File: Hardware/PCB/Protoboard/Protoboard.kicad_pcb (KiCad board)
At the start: 2 copper layers, 17 parts, among them J1 Conn_01x05_Female, J2 Conn_01x08_Female, J3 Conn_01x08_Female, U1 MAX6971ANG_

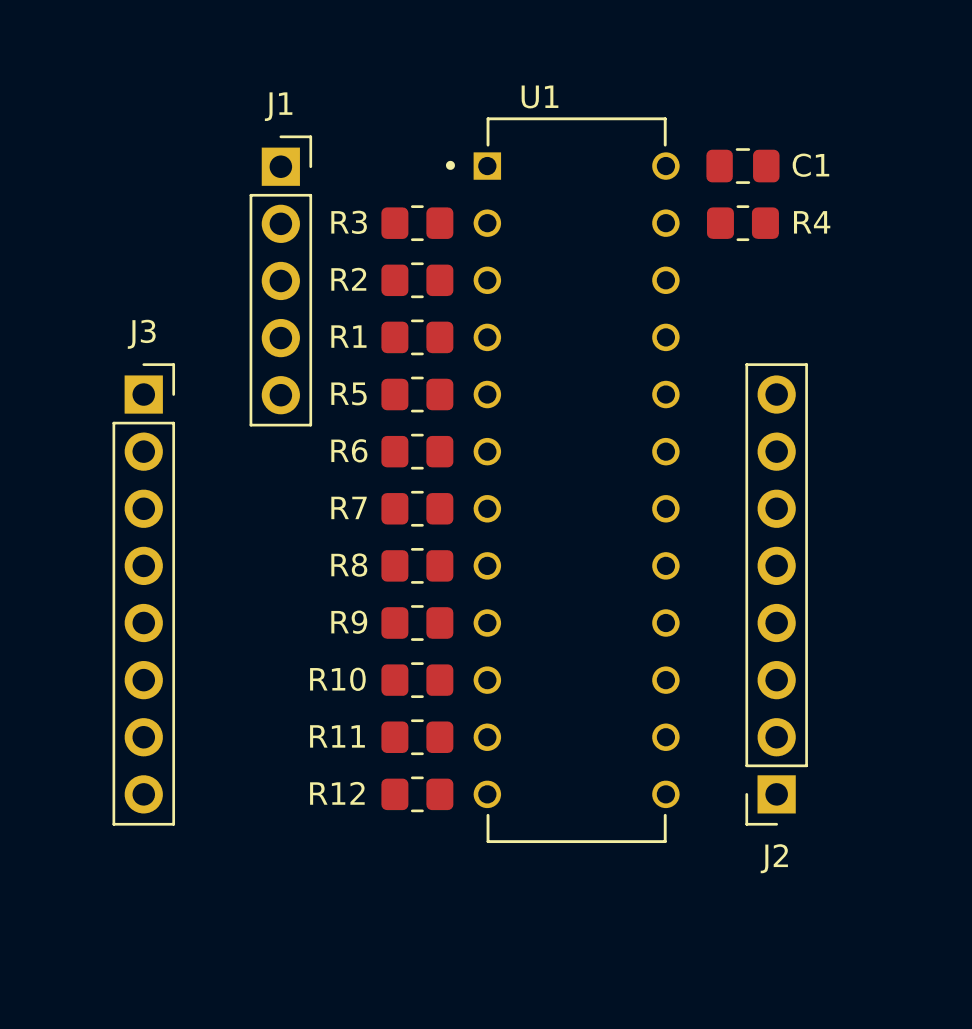
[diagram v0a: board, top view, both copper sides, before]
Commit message: Finished Protoboard
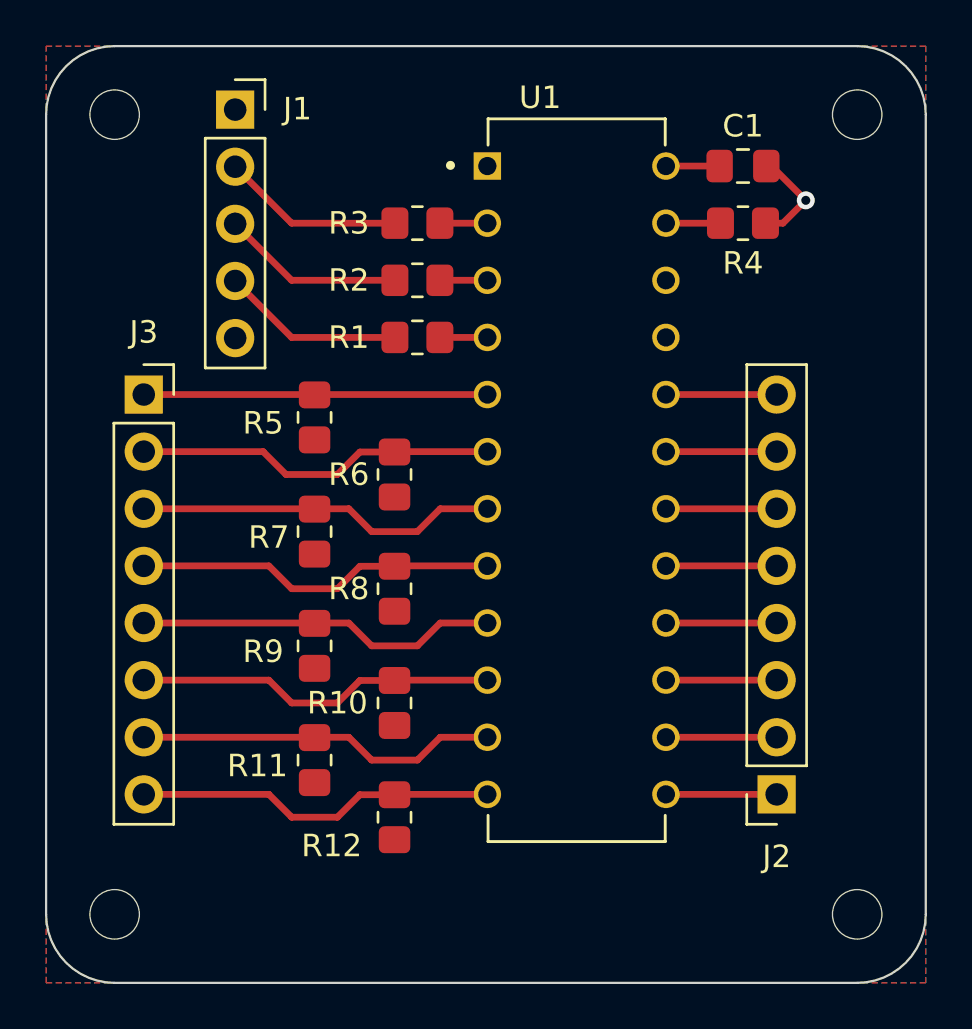
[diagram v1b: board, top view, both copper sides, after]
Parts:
- added H1: MountingHole, MountingHole:MountingHole_2.2mm_M2, F.Cu at (119.4, 68.6)
- added H2: MountingHole, MountingHole:MountingHole_2.2mm_M2, F.Cu at (152.4, 68.6)
- added H3: MountingHole, MountingHole:MountingHole_2.2mm_M2, F.Cu at (152.4, 104.1)
- added H4: MountingHole, MountingHole:MountingHole_2.2mm_M2, F.Cu at (119.4, 104.1)
- moved R5 4.68 mm to (128.3, 82.0), turned to 90 degrees
- moved R7 4.68 mm to (128.3, 87.1), turned to 90 degrees
- moved R11 4.68 mm to (128.3, 97.3), turned to 90 degrees
- moved R9 4.68 mm to (128.3, 92.2), turned to 90 degrees
- moved J1 3.25 mm to (124.7, 68.4)
- moved R10 1.44 mm to (131.8, 94.7), turned to 90 degrees
- moved R12 1.44 mm to (131.8, 99.8), turned to 90 degrees
- moved R8 1.44 mm to (131.8, 89.7), turned to 90 degrees
- moved R6 1.44 mm to (131.8, 84.6), turned to 90 degrees
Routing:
- net Net-(J3-Pad7): track 0.00 -> 16.1 mm
- net Net-(J3-Pad3): track 0.00 -> 16.1 mm
- net Net-(J3-Pad5): track 0.00 -> 16.1 mm
- net Net-(J3-Pad6): track 0.00 -> 16.1 mm
- net Net-(J3-Pad8): track 0.00 -> 16.1 mm
- net Net-(J3-Pad4): track 0.00 -> 16.1 mm
- net Net-(J3-Pad2): track 0.00 -> 16.1 mm
- net Net-(J3-Pad1): track 0.00 -> 15.3 mm
- net Net-(J1-Pad4): track 0.00 -> 8.14 mm
- net Net-(J1-Pad2): track 0.00 -> 8.14 mm
- net Net-(J1-Pad3): track 0.00 -> 8.14 mm
- net Net-(J2-Pad8): track 0.00 -> 4.93 mm
- net Net-(J2-Pad7): track 0.00 -> 4.93 mm
- net Net-(J2-Pad6): track 0.00 -> 4.93 mm
- net Net-(J2-Pad5): track 0.00 -> 4.93 mm
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- added copper zone on B.Cu, net GND
- added copper zone on F.Cu, net VCC
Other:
- board outline added: 39.1 x 41.7 mm
